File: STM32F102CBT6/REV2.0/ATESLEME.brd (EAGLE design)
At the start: 35.3 x 57.9 mm, 65 parts, among them U1 ADXL345PATRICK, U2 MS561101BA03-50, U3 AMS1117-3.3, U4 STM32F102CBT6, U5 38kHz, X1 JST-XH-04-PIN-LONG-PAD, Y2 ABM2B-8.000MHZ-10-1-U-T

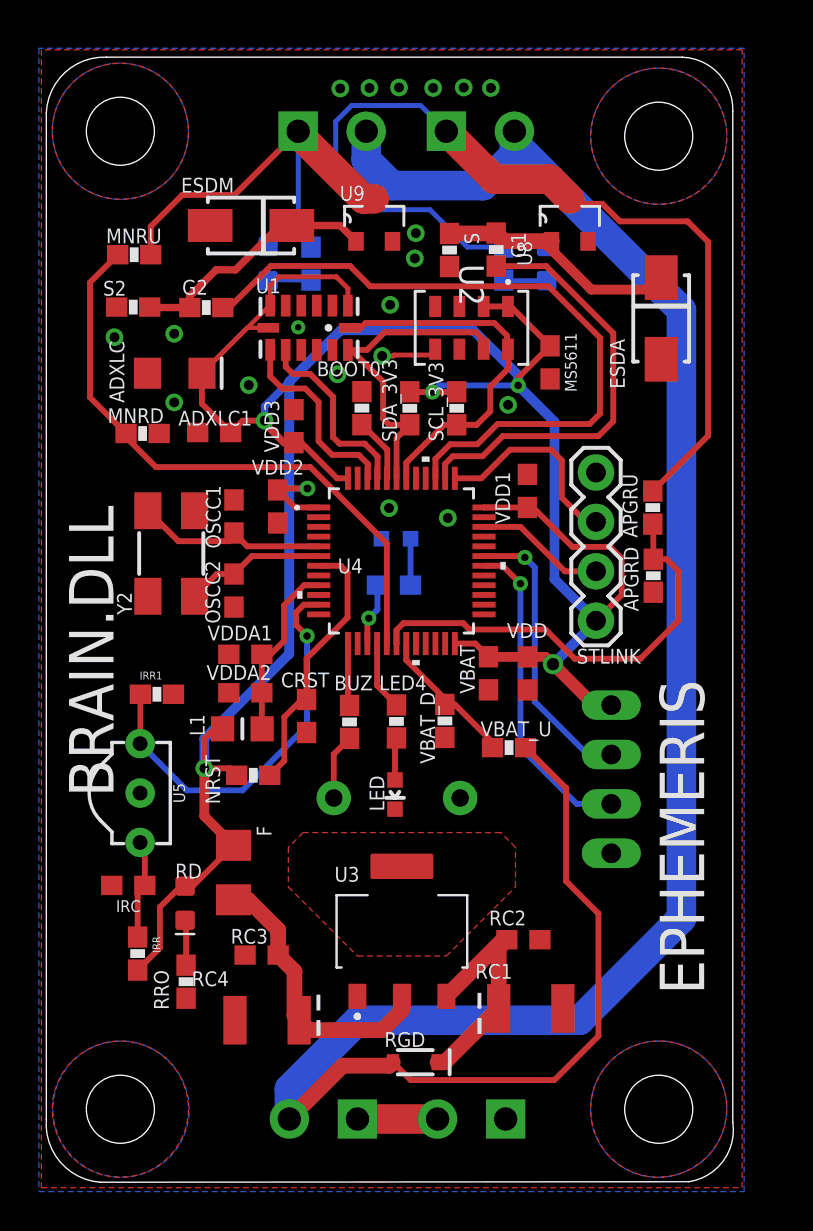
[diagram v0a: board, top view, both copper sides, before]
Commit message: Version 2.0 was updated by brain.dll
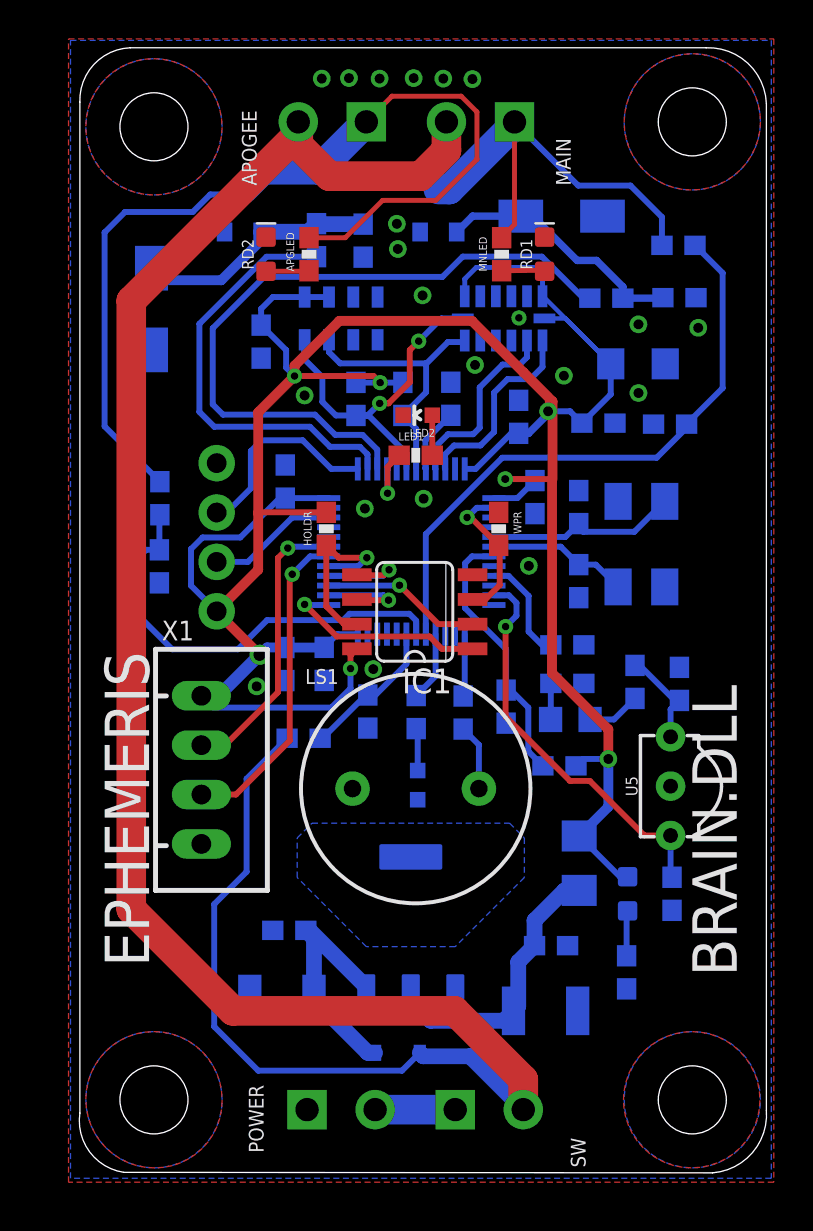
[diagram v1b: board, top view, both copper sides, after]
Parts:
- added HOLDR, WPR: 10k, SparkFun-Resistors:0603-RES
- added IC1: WS2811-SOP8, adafruit:SO08-SKINNYPADS
- moved IRC 30.2 mm to (33.3, 26.6), flipped to the bottom, turned to 90 degrees
- moved IRR 29.1 mm to (31.0, 26.7), flipped to the bottom
- moved IRR1 28.4 mm to (32.9, 15.8), flipped to the bottom, turned to 270 degrees
- moved S2 28.1 mm to (33.3, 46.5), flipped to the bottom
- moved MNRU 28.0 mm to (33.2, 49.2), flipped to the bottom
- moved U5 27.3 mm to (32.8, 21.4), turned to 90 degrees
- moved MNRD 27.1 mm to (32.8, 40.0), flipped to the bottom
- moved ESDA 26.2 mm to (6.15, 45.9), flipped to the bottom
- moved APGRD 25.4 mm to (6.55, 32.7), flipped to the bottom
- moved APGRU 25.4 mm to (6.58, 36.2), flipped to the bottom
- moved Y2 24.2 mm to (31.3, 33.8), flipped to the bottom
- moved ADXLC 23.8 mm to (31.2, 43.1), flipped to the bottom
- moved RD 22.8 mm to (30.6, 15.8), flipped to the bottom
- moved RRO 22.7 mm to (30.6, 11.8), flipped to the bottom
- moved X1 21.1 mm to (8.71, 22.2), flipped to the top
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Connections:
- removed net PC13: U4.2
- new net CS: IC1.1, U4.25
- new net HOLD: HOLDR.1, IC1.7, U4.29
- new net MISO: IC1.2, U4.27
- new net MOSI: IC1.5, U4.28
- new net SCK: IC1.6, U4.26
- new net WP: IC1.3, U4.2, WPR.2
- net 3.3V: now also HOLDR.2, IC1.8
- net GND: now also IC1.4, WPR.1
- net LED2: now also U4.40; no longer U4.15
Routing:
- net 3.3V: track 140.5 -> 154.3 mm, vias 6 -> 7
- net CS: track 0.00 -> 10.8 mm, vias 0 -> 1
- net HOLD: track 0.00 -> 9.58 mm, vias 0 -> 1
- net MISO: track 0.00 -> 8.24 mm, vias 0 -> 1
- net WP: track 0.00 -> 7.57 mm, vias 0 -> 1
- net MOSI: track 0.00 -> 5.01 mm, vias 0 -> 1
- net SCK: track 0.00 -> 4.83 mm, vias 0 -> 1
- net GND: track 2.89 -> 0.00 mm, vias 19 -> 21
- net SDA_3V3: track 16.9 -> 14.5 mm
- net SCL_3V3: track 19.1 -> 18.4 mm, vias 0 -> 2
- added copper zone on layer 16, net HT
- removed copper zone on layer 1, net HT
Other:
- outline, holes or cut-outs redrawn
